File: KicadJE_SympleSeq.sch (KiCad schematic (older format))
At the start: 18 parts

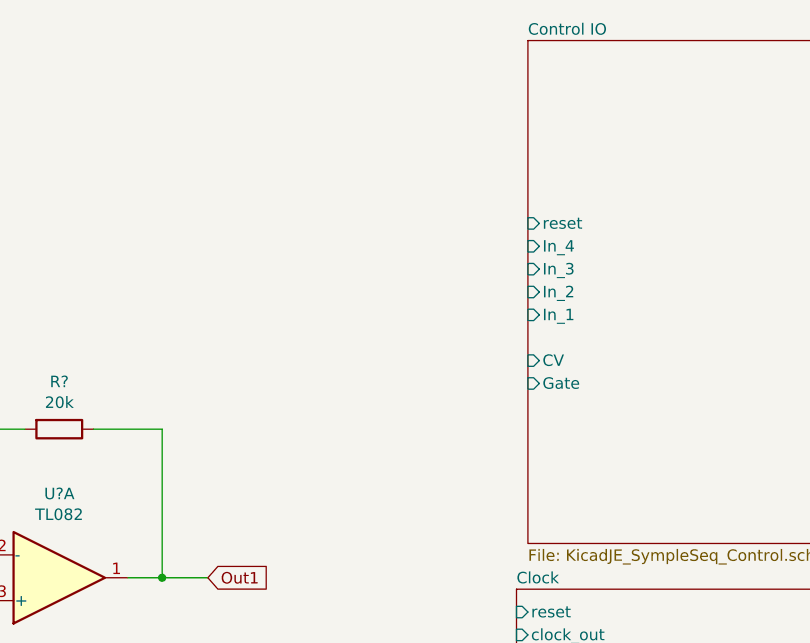
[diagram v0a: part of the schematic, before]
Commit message: Sch taking form
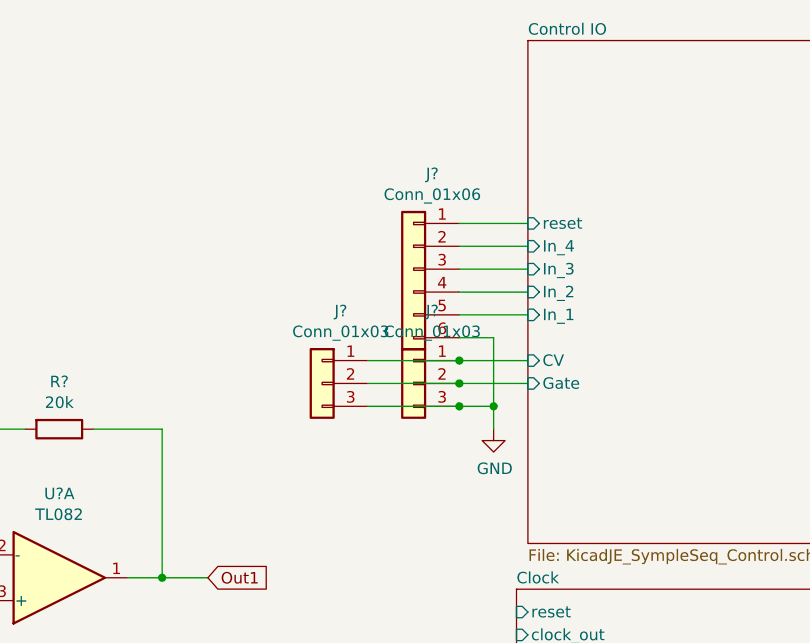
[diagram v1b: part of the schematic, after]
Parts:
- added J?: Conn_01x06, symbol Connector_Generic:Conn_01x06
- added J? (x2): Conn_01x03, symbol Connector_Generic:Conn_01x03
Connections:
- net Control IO/CV: now also J?.1 (Pin_1), J?.1 (Pin_1)
- net Control IO/Gate: now also J?.2 (Pin_2), J?.2 (Pin_2)
- net Control IO/In_1: now also J?.5 (Pin_5)
- net Control IO/In_2: now also J?.4 (Pin_4)
- net Control IO/In_3: now also J?.3 (Pin_3)
- net Control IO/In_4: now also J?.2 (Pin_2)
- net Control IO/reset: now also J?.1 (Pin_1)
- net GND: now also J?.3 (Pin_3), J?.3 (Pin_3), J?.6 (Pin_6)
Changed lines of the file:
@@
 Wire Wire Line
 	1800 5500 1800 6100
+$Comp
+L Connector_Generic:Conn_01x06 J?
+U 1 1 5DAE9349
+P 6500 3600
+F 0 "J?" H 6418 4017 50  0000 C CNN
+F 1 "Conn_01x06" H 6418 3926 50  0000 C CNN
+F 2 "" H 6500 3600 50  0001 C CNN
+F 3 "~" H 6500 3600 50  0001 C CNN
+	1    6500 3600
+	-1   0    0    -1
+$EndComp
+$Comp
+L Connector_Generic:Conn_01x03 J?
+U 1 1 5DAEAEAF
+P 6500 4100
+F 0 "J?" H 6418 4417 50  0000 C CNN
+F 1 "Conn_01x03" H 6418 4326 50  0000 C CNN
+F 2 "" H 6500 4100 50  0001 C CNN
+F 3 "~" H 6500 4100 50  0001 C CNN
+	1    6500 4100
+	-1   0    0    -1
+$EndComp
+$Comp
+L Connector_Generic:Conn_01x03 J?
+U 1 1 5DAEBA5E
+P 6100 4100
+F 0 "J?" H 6018 4417 50  0000 C CNN
+F 1 "Conn_01x03" H 6018 4326 50  0000 C CNN
+F 2 "" H 6100 4100 50  0001 C CNN
+F 3 "~" H 6100 4100 50  0001 C CNN
+	1    6100 4100
+	-1   0    0    -1
+$EndComp
+Wire Wire Line
+	6700 4000 7000 4000
+Wire Wire Line
+	6700 4100 7000 4100
+Wire Wire Line
+	6700 3800 7000 3800
+Wire Wire Line
+	6700 3700 7000 3700
+Wire Wire Line
+	6700 3600 7000 3600
+Wire Wire Line
+	6700 3500 7000 3500
+Wire Wire Line
+	6700 3400 7000 3400
+Wire Wire Line
+	6300 4000 6700 4000
+Connection ~ 6700 4000
+Wire Wire Line
+	6300 4100 6700 4100
+Connection ~ 6700 4100
+Wire Wire Line
+	6300 4200 6700 4200
+$Comp
+L Envelope-cache-2018-08-04-13-00-04:GND #PWR?
+U 1 1 5DAF76B5
+P 6850 4300
+AR Path="/5DAF76B5" Ref="#PWR?"  Part="1"
+AR Path="/5C8C5FC0/5DAF76B5" Ref="#PWR?"  Part="1"
+F 0 "#PWR?" H 6850 4050 50  0001 C CNN
+F 1 "GND" H 6855 4127 50  0000 C CNN
+F 2 "" H 6850 4300 50  0001 C CNN
+F 3 "" H 6850 4300 50  0001 C CNN
+	1    6850 4300
+	1    0    0    -1
+$EndComp
+Wire Wire Line
+	6700 4200 6850 4200
+Wire Wire Line
+	6850 4200 6850 4300
+Connection ~ 6700 4200
+Wire Wire Line
+	6700 3900 6850 3900
+Wire Wire Line
+	6850 3900 6850 4200
+Connection ~ 6850 4200
 $EndSCHEMATC

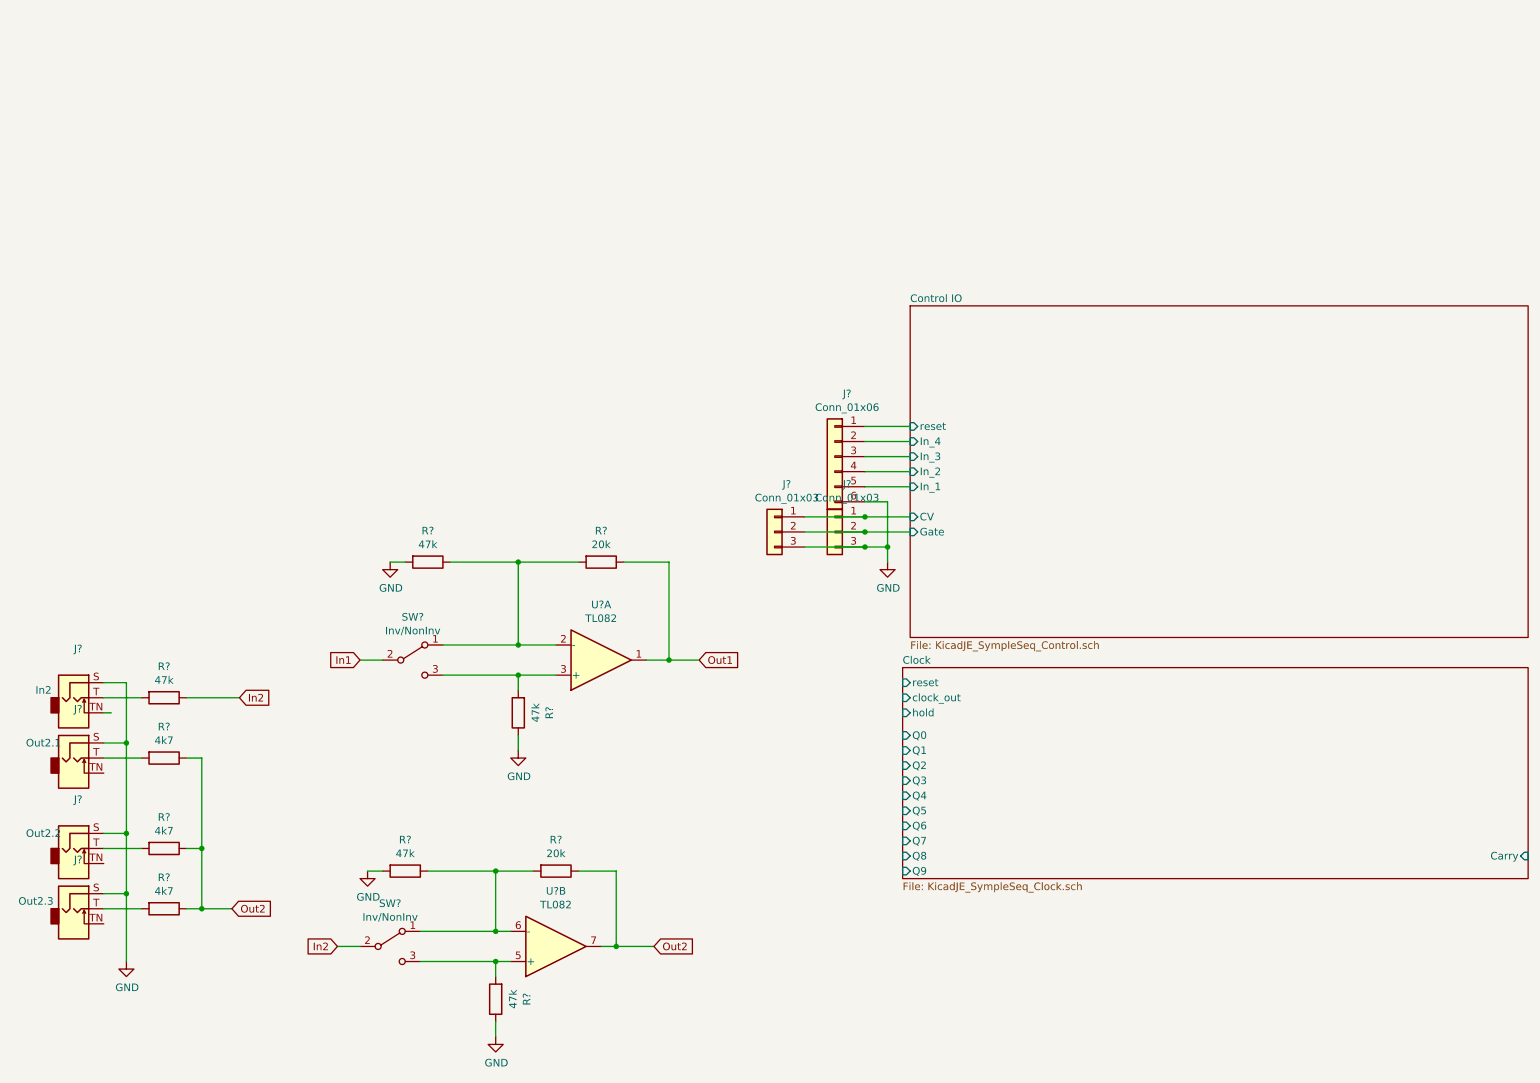
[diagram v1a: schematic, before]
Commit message: pin headers
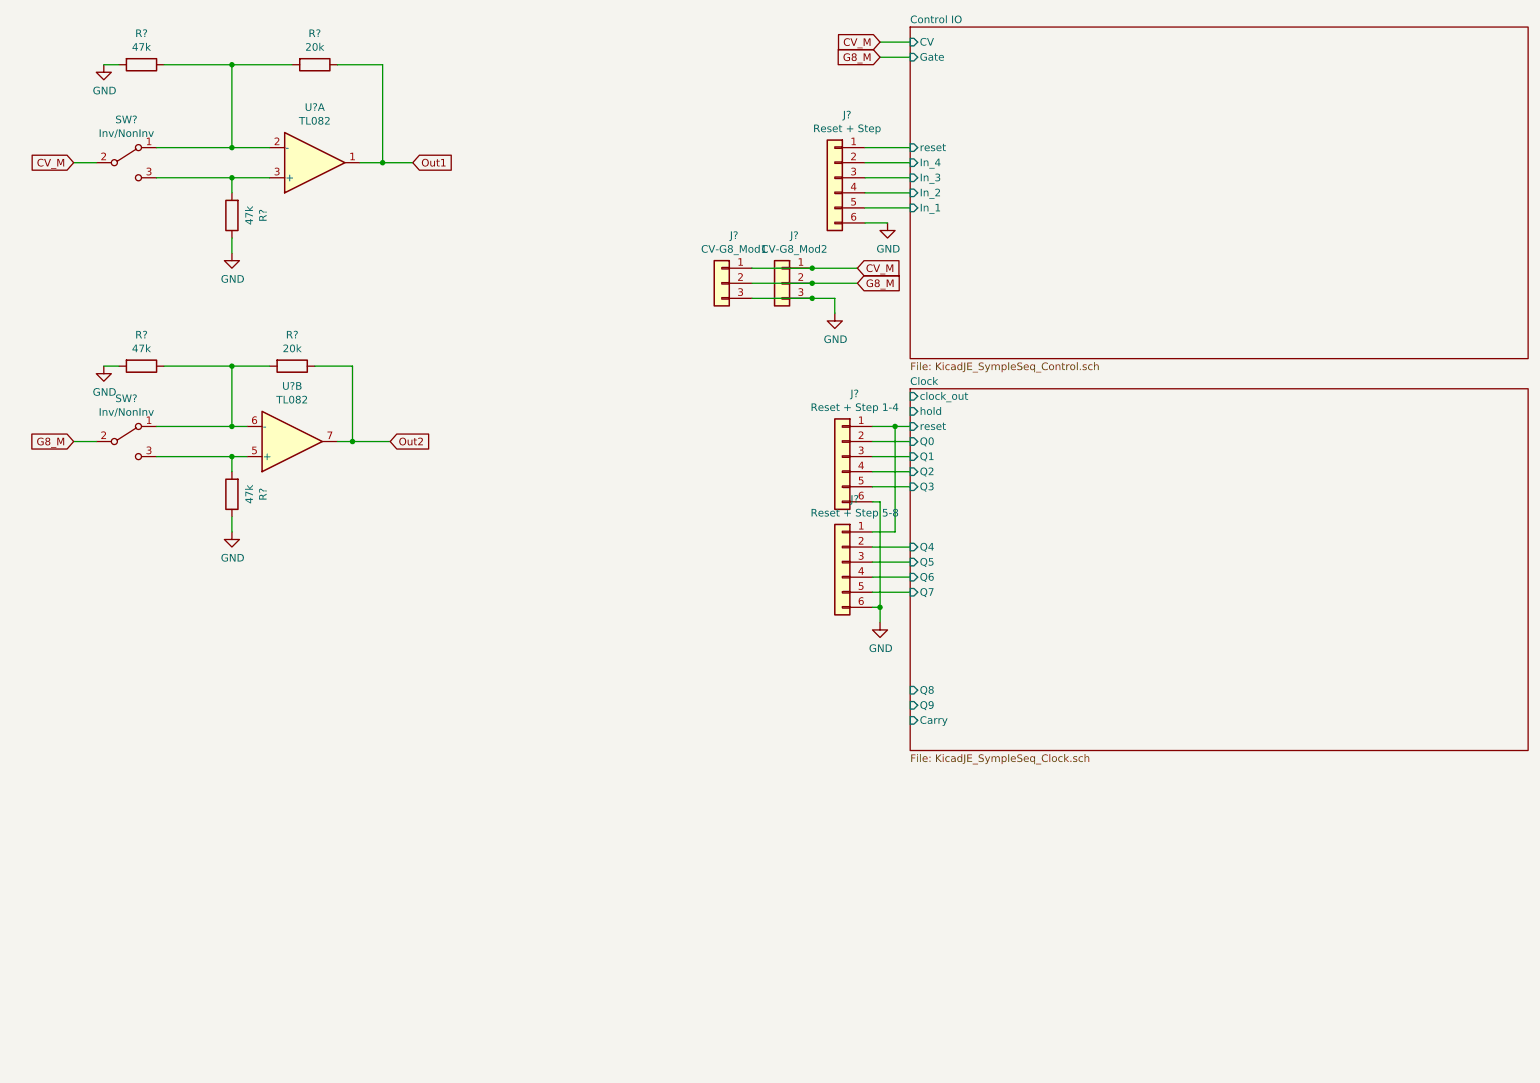
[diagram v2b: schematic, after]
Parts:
- removed J?: In2, AJ-Dropbox-Kicad:PJ301SM, symbol Connector:AudioJack2_SwitchT
- removed J?: Out2.1, AJ-Dropbox-Kicad:PJ301SM, symbol Connector:AudioJack2_SwitchT
- removed J?: Out2.3, AJ-Dropbox-Kicad:PJ301SM, symbol Connector:AudioJack2_SwitchT
- removed J?: Out2.2, AJ-Dropbox-Kicad:PJ301SM, symbol Connector:AudioJack2_SwitchT
- removed R?: 47k, Resistor_SMD:R_0805_2012Metric_Pad1.15x1.40mm_HandSolder, symbol Device:R
- removed R? (x3): 4k7, Resistor_SMD:R_0805_2012Metric_Pad1.15x1.40mm_HandSolder, symbol Device:R
- added J?: Reset + Step 1-4, symbol Connector_Generic:Conn_01x06
- added J?: Reset + Step 5-8, symbol Connector_Generic:Conn_01x06
- J?: value Conn_01x06 -> Reset + Step
- J?: value Conn_01x03 -> CV-G8_Mod2
- J?: value Conn_01x03 -> CV-G8_Mod1
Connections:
- net In1 is gone; now on net CV_M: SW?.2 (B)
- net In2 is gone; now on net G8_M: SW?.2 (B)
- net Clock/Q0: now also J?.2 (Pin_2)
- net Clock/Q1: now also J?.3 (Pin_3)
- net Clock/Q2: now also J?.4 (Pin_4)
- net Clock/Q3: now also J?.5 (Pin_5)
- net Clock/Q4: now also J?.2 (Pin_2)
- net Clock/Q5: now also J?.3 (Pin_3)
- net Clock/Q6: now also J?.4 (Pin_4)
- net Clock/Q7: now also J?.5 (Pin_5)
- net Clock/reset: now also J?.1 (Pin_1), J?.1 (Pin_1)
- net GND: now also J?.6 (Pin_6), J?.6 (Pin_6)
- net Control IO/CV renamed CV_M
- net Control IO/Gate renamed G8_M
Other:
- moved on the sheet: J?, R?, SW?, U?A, U?B

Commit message: base circuit done
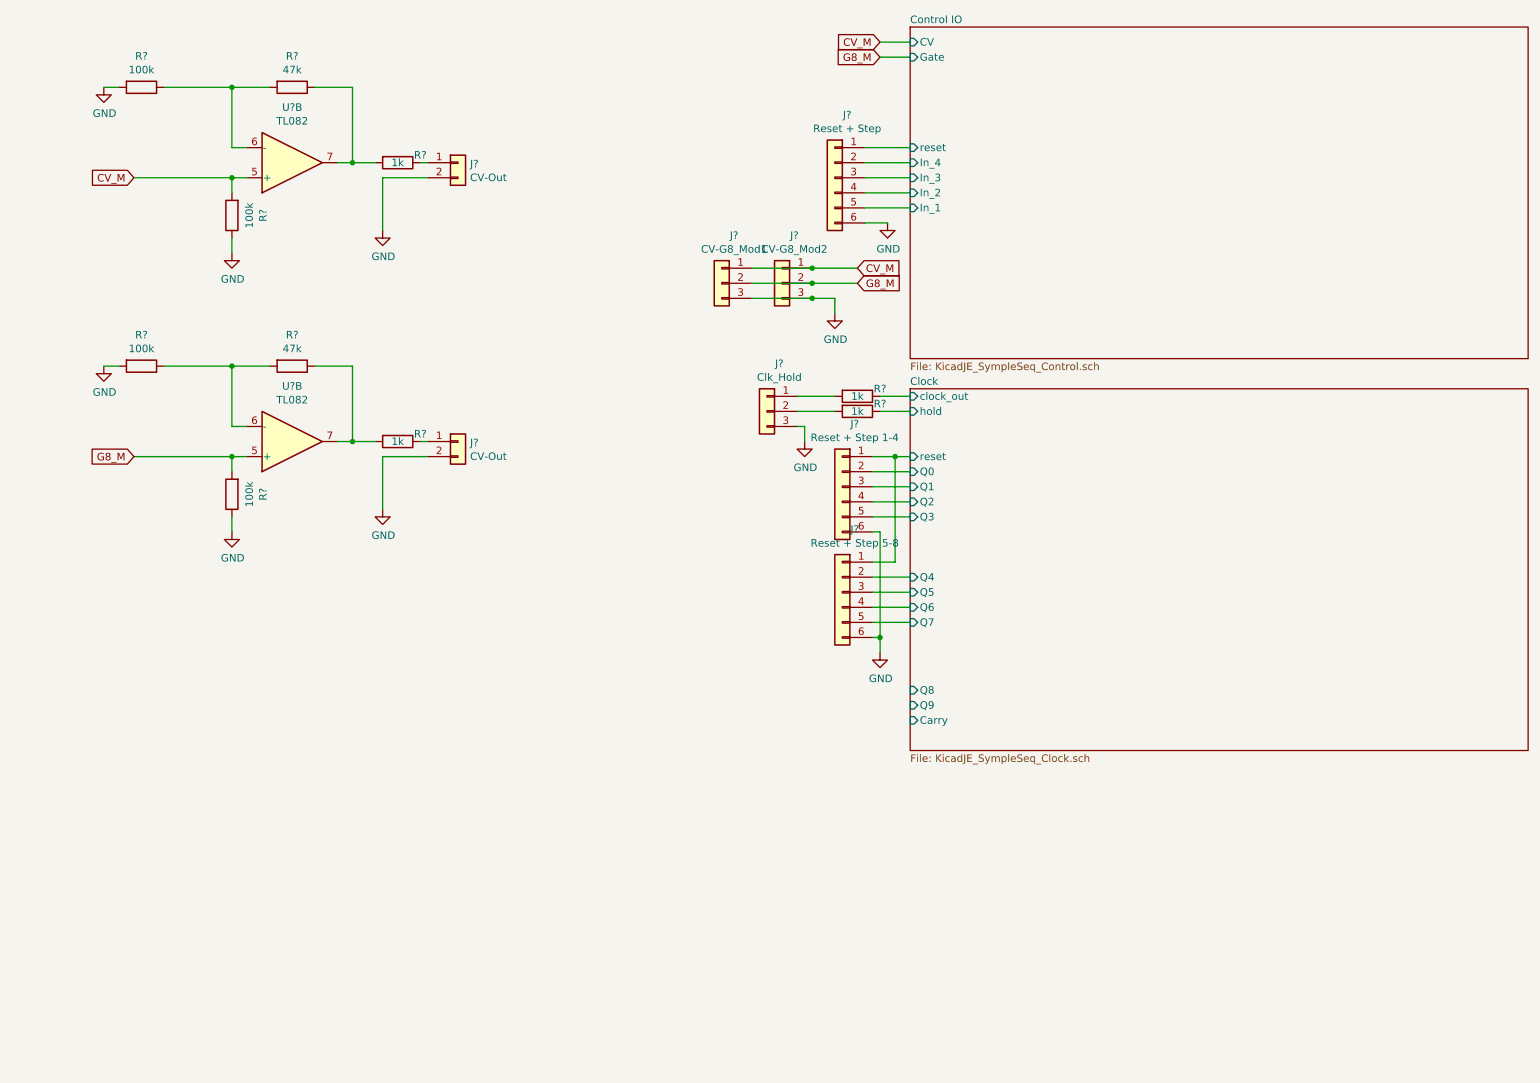
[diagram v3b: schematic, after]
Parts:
- removed R?: 20k, Resistor_SMD:R_0805_2012Metric_Pad1.15x1.40mm_HandSolder, symbol Device:R
- removed R? (x2): 47k, Resistor_SMD:R_0805_2012Metric_Pad1.15x1.40mm_HandSolder, symbol Device:R
- removed SW? (x2): Inv/NonInv, AJ-Dropbox-Kicad:SP1MS1, symbol Switch:SW_SPDT
- removed U?: TL082, AJ-Dropbox-Kicad:AJ_SO-8_5.3x6.2mm_P1.27mm, symbol Amplifier_Operational:TL082
- added J?: Clk_Hold, symbol Connector_Generic:Conn_01x03
- added J? (x2): CV-Out, symbol Connector_Generic:Conn_01x02
- added R? (x4): 1k, Resistor_SMD:R_0805_2012Metric_Pad1.15x1.40mm_HandSolder, symbol Device:R
- added R?: 47k, Resistor_SMD:R_0805_2012Metric_Pad1.15x1.40mm_HandSolder, symbol Device:R
- added R? (x2): 100k, Resistor_SMD:R_0805_2012Metric_Pad1.15x1.40mm_HandSolder, symbol Device:R
- added U?: TL082, symbol Amplifier_Operational:TL082
- R?: value 20k -> 47k
- R? (x2): value 47k -> 100k
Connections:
- net CV_M: now also R?.2, U?.5 (+)
- net Clock/clock_out: now also R?.1
- net Clock/hold: now also R?.1
- net G8_M: now also R?.2, U?.5 (+)
- net GND: now also J?.2 (Pin_2), J?.2 (Pin_2), J?.3 (Pin_3), R?.1, R?.2
- net Out2: no longer names the net of R?.1, U?.7
- net Out2: now also R?.2
- new net: J?.1 (Pin_1), R?.2
- new net: J?.2 (Pin_2), R?.2
- new net: J?.1 (Pin_1), R?.1 (x2)
- new net: R?.1, R?.2, U?.6 (-)
- new net: R?.1, R?.2, U?.7
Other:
- moved on the sheet: J?
